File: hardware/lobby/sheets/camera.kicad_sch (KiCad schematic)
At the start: 3 parts, among them J4 Conn_01x22_Female

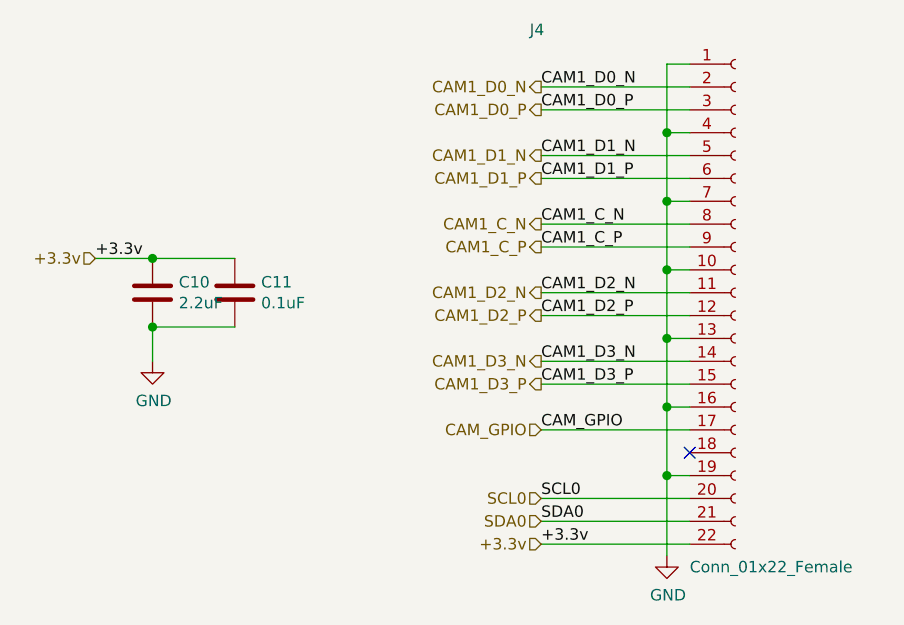
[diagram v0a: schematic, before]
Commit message: update lobby
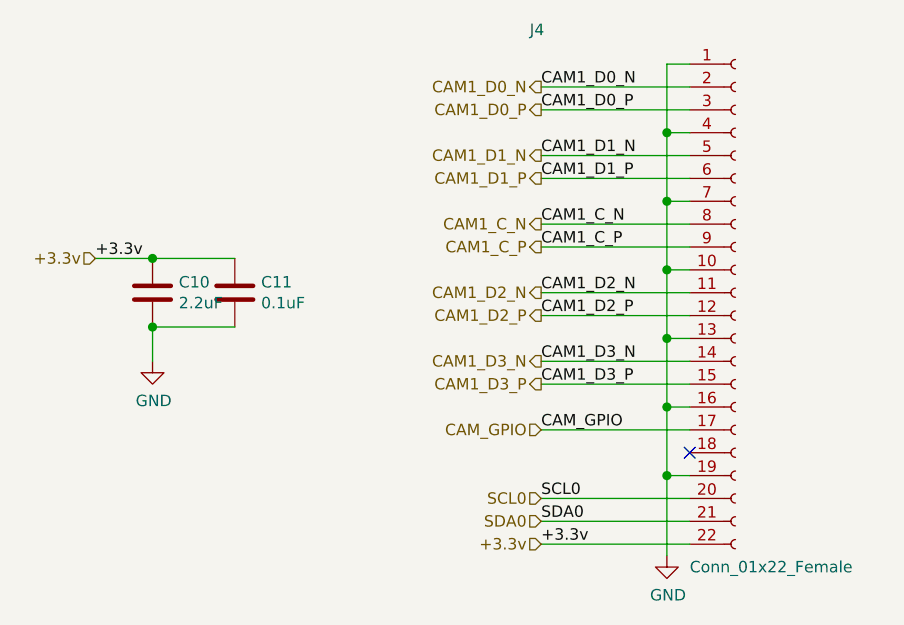
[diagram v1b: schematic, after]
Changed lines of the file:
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@@
   (symbol (lib_id "power:GND") (at 88.9 91.44 0) (unit 1)
     (in_bom yes) (on_board yes)
-    (property "Reference" "#PWR0101" (id 0) (at 88.9 97.79 0)
+    (property "Reference" "#PWR0100" (id 0) (at 88.9 97.79 0)
       (effects (font (size 1.27 1.27)) hide)
     )
@@
   (symbol (lib_id "power:GND") (at 146.05 113.03 0) (unit 1)
     (in_bom yes) (on_board yes)
-    (property "Reference" "#PWR0102" (id 0) (at 146.05 119.38 0)
+    (property "Reference" "#PWR0101" (id 0) (at 146.05 119.38 0)
       (effects (font (size 1.27 1.27)) hide)
     )
@@
       (effects (font (size 1.27 1.27)) hide)
     )
-    (property "Datasheet" "https://search.murata.co.jp/Ceramy/image/img/A01X/G101/ENG/GRM21BR71A106KA73-01.pdf" (id 3) (at 88.9 83.82 0)
+    (property "Datasheet" "~" (id 3) (at 88.9 83.82 0)
       (effects (font (size 1.27 1.27)) hide)
     )
@@
       (effects (font (size 1.27 1.27)) hide)
     )
-    (property "Datasheet" "https://search.murata.co.jp/Ceramy/image/img/A01X/G101/ENG/GRM21BR71A106KA73-01.pdf" (id 3) (at 98.044 83.82 0)
+    (property "Datasheet" "~" (id 3) (at 98.044 83.82 0)
       (effects (font (size 1.27 1.27)) hide)
     )
@@
       (effects (font (size 1.27 1.27)) hide)
     )
-    (property "Datasheet" "https://www.hirose.com/product/document?clcode=&productname=&series=FH12&documenttype=Catalog&lang=en&documentid=D31648_en" (id 3) (at 153.67 83.82 0)
+    (property "Datasheet" "~" (id 3) (at 153.67 83.82 0)
       (effects (font (size 1.27 1.27)) hide)
     )
